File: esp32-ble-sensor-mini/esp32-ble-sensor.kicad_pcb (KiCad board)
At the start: 2 copper layers, 39 x 54 mm, 39 parts, among them J1 Conn_01x08_Pin, J4 USB4215-03-A_REVA, SW1 SW_SPST, SW2 SW_SPST, SW3 SW_SPST, U1 ESP32-C6-MINI-1/U, U2 SHT4x, U3 TPD4E05U06DQA, U4 SCD41-D-R2, U5 TLV75533PDYDR, U6 LM66200DRLR

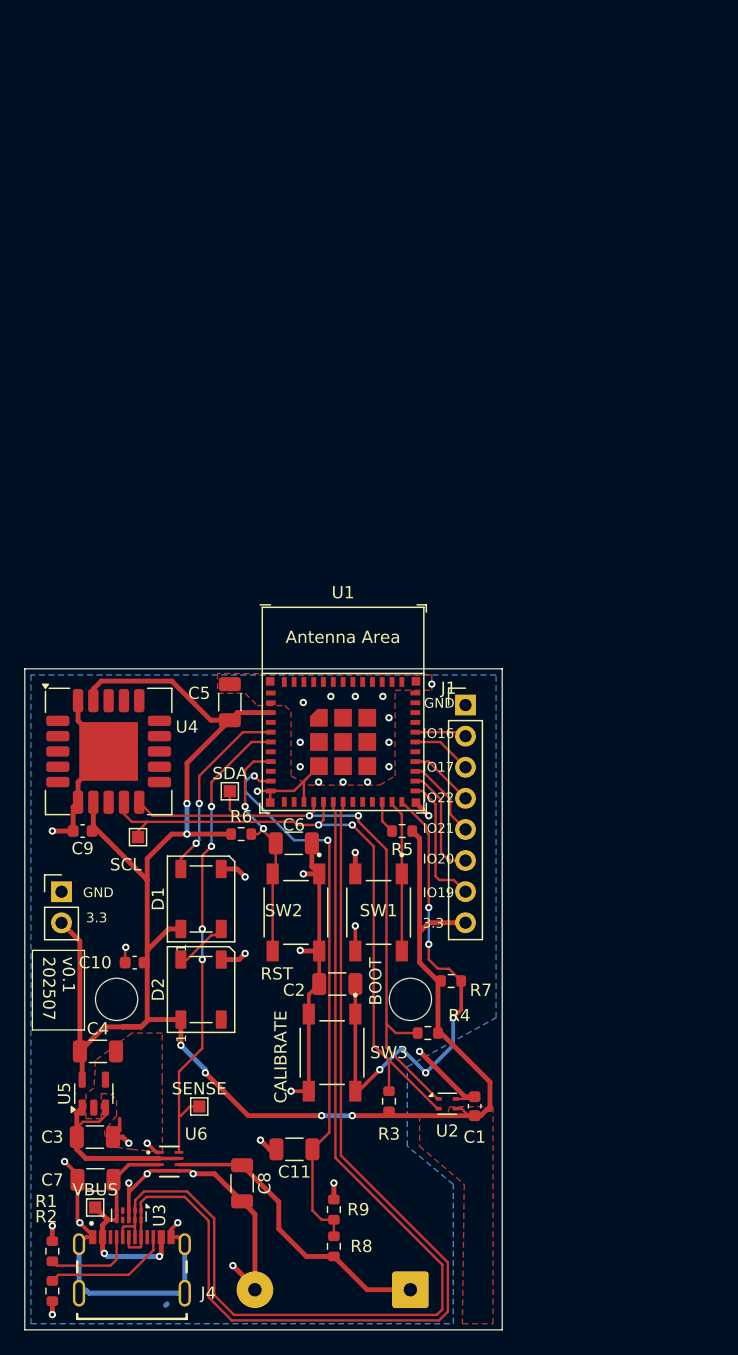
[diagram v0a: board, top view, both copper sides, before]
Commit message: esp32 sensor 202509
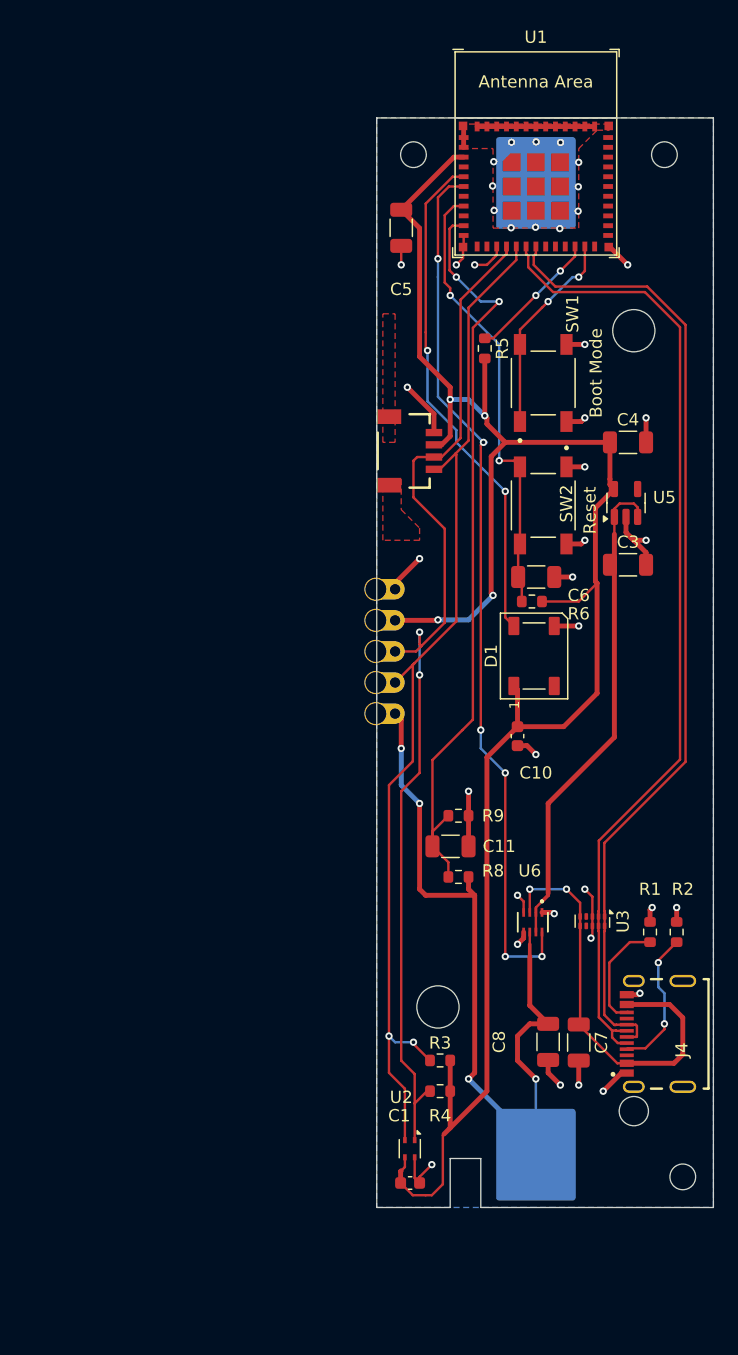
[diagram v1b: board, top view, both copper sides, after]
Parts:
- removed C2: 1uF, Capacitor_SMD:C_1206_3216Metric
- removed C9: 100nF, Capacitor_SMD:C_0603_1608Metric
- removed D2: WS2812B, LED_SMD:LED_WS2812B_PLCC4_5.0x5.0mm_P3.2mm
- removed J1: Conn_01x08_Pin, Connector_PinHeader_2.54mm:PinHeader_1x08_P2.54mm_Vertical
- removed R7: 10k, Resistor_SMD:R_0603_1608Metric
- removed the REF** at (119.2, 103.2)
- removed SCL, SDA, SENSE, VBUS: TestPoint_Pad_1.0x1.0mm, TestPoint:TestPoint_Pad_1.0x1.0mm
- removed SW3: SW_SPST, Library:SW_TS18-5-17-SL-260-SMT-TR
- removed U4: SCD41-D-R2, Sensor:Sensirion_SCD4x-1EP_10.1x10.1mm_P1.25mm_EP4.8x4.8mm
- added J2: Qwiic_RA, SparkFun-Connector:JST_SMD_1.0mm-4_Black, F.Cu at (149.7, 67.2)
- added J3: Conn_01x05, SparkFun-Connector:1x05_Castellated, B.Cu at (146.5, 78.5)
- added REF**: MountingHole_2.1mm, MountingHole:MountingHole_2.1mm, F.Cu at (148.0, 43.0)
- added REF**: MountingHole_2.1mm, MountingHole:MountingHole_2.1mm, F.Cu at (168.5, 43.0)
- added REF**: MountingHole_2.1mm, MountingHole:MountingHole_2.1mm, F.Cu at (170.0, 126.5)
- BT1: footprint Battery:BatteryHolder_Keystone_2479_3xAAA -> Battery:BatteryHolder_Keystone_1042_1x18650
- moved C4 66.0 mm to (165.5, 66.5)
- moved U5 64.9 mm to (165.4, 71.5)
- moved C3 63.9 mm to (165.5, 76.5)
- moved R1 57.3 mm to (169.5, 106.5)
- moved R2 57.0 mm to (167.3, 106.5), turned to -90 degrees
- moved BT1 51.7 mm to (158.0, 85.0)
- moved J4 49.7 mm to (170.0, 114.8), turned to 90 degrees
- moved U1 48.0 mm to (158.0, 42.9)
- moved SW1 45.3 mm to (158.6, 61.6), turned to 90 degrees
- moved U3 44.8 mm to (162.6, 105.6)
- moved C5 41.2 mm to (147.0, 49.0), turned to 90 degrees
- moved C7 41.0 mm to (161.5, 115.5), turned to -90 degrees
- moved R5 40.0 mm to (153.8, 58.8), turned to -90 degrees
- moved SW2 38.9 mm to (158.6, 71.7)
- moved C10 36.3 mm to (156.5, 90.5), turned to -90 degrees
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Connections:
- D1 pad 2: Net-(D1-DOUT) -> unconnected-(D1-DOUT-Pad2)
- U1 pad 24: Net-(SW3-A) -> unconnected-(U1-GPIO18-Pad24)
- U1 pad 25: Net-(J1-Pin_7) -> unconnected-(U1-GPIO19-Pad25)
- U1 pad 26: Net-(J1-Pin_6) -> unconnected-(U1-GPIO20-Pad26)
- U1 pad 27: Net-(J1-Pin_5) -> unconnected-(U1-GPIO21-Pad27)
- U1 pad 28: Net-(J1-Pin_4) -> unconnected-(U1-GPIO22-Pad28)
- U1 pad 30: Net-(J1-Pin_3) -> unconnected-(U1-U0RXD/GPIO17-Pad30)
- U1 pad 31: Net-(J1-Pin_2) -> unconnected-(U1-U0TXD/GPIO16-Pad31)
- U5 pad 4: GND -> unconnected-(U5-NR-Pad4)
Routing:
- net GND: track 130.3 -> 75.3 mm, vias 38 -> 40
- net Net-(SW3-A): track 42.7 -> 0.00 mm, vias 5 -> 0
- net Net-(BT1-+): track 24.5 -> 66.6 mm, vias 0 -> 4
- net /SDA: track 51.0 -> 87.0 mm
- net /POWER_SENSE: track 39.5 -> 72.2 mm, vias 4 -> 6
- net /SCL: track 54.6 -> 86.6 mm
- net Net-(D1-DIN): track 15.6 -> 41.5 mm
- net /500ma Power Supply (page 2)/VIN: track 17.4 -> 40.3 mm
- net /CHIP_PU: track 19.5 -> 36.8 mm
- net /VBUS: track 19.0 -> 35.9 mm
- net /VBAT_SENSE: track 45.9 -> 62.6 mm
- net +3.3V: track 146.2 -> 160.4 mm, vias 6 -> 4
- net Net-(J1-Pin_7): track 11.0 -> 0.00 mm
- net Net-(J1-Pin_6): track 9.32 -> 0.00 mm
- net /BOOT_MODE_SEL: track 2.71 -> 11.0 mm, vias 0 -> 2
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- added copper zone on F.Cu, net unconnected-(J2-NC-PadNC1)
- added copper zone on F.Cu, net unconnected-(J2-NC-PadNC2)
- removed copper zone on F.Cu, net +3.3V
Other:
- board size 39 x 54 mm -> 27.5 x 89 mm
- board text added: "+"
- board text added: "Boot Mode"
- board text added: "ESP Sensor 202509"
- board text added: "Reset"
- board text removed: "3.3"
- board text removed: "BOOT"
- board text removed: "CALIBRATE"
- board text removed: "GND"
- board text removed: "IO16"
- board text removed: "IO17"
- board text removed: "IO19"
- board text removed: "IO20"
- board text removed: "IO21"
- board text removed: "IO22"
- board text removed: "RST"
- board text removed: "v0.1 202507"
